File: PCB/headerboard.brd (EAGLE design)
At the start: 100 x 80 mm, 21 parts

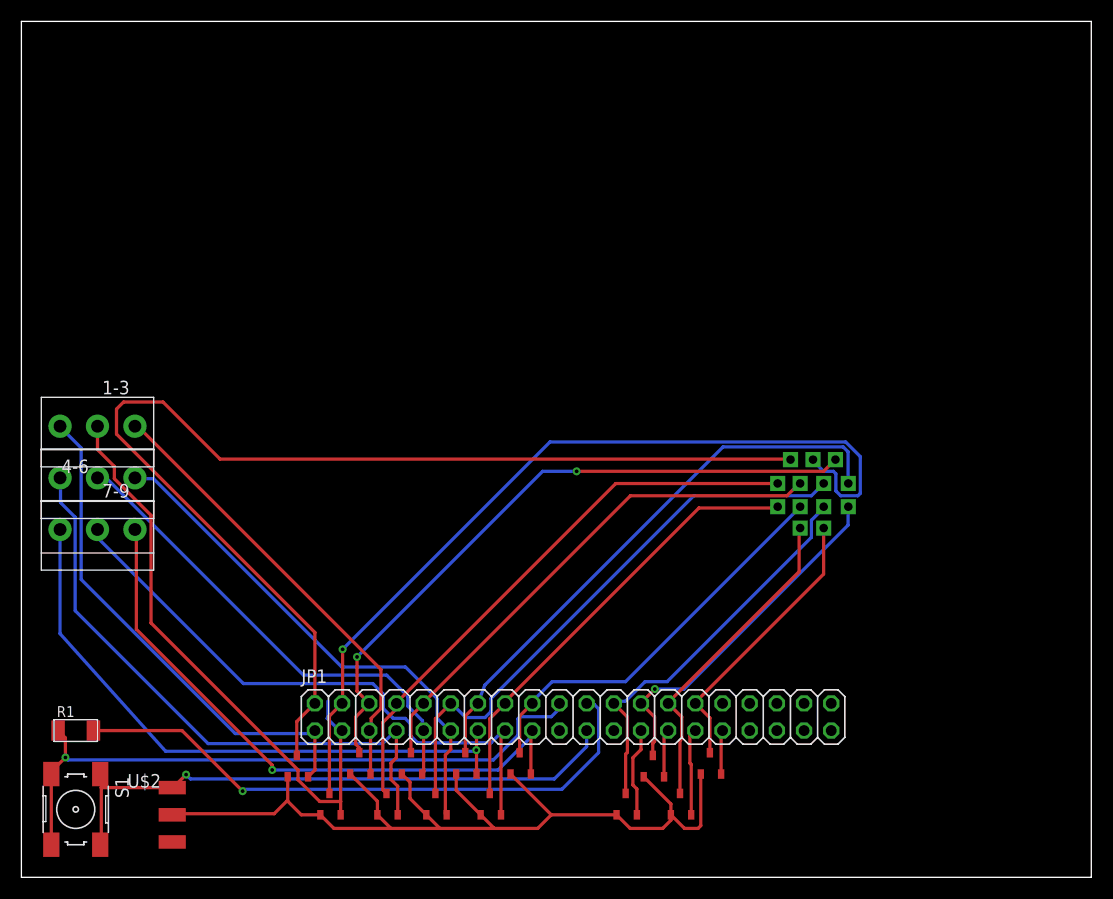
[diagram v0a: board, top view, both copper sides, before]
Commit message: Updates
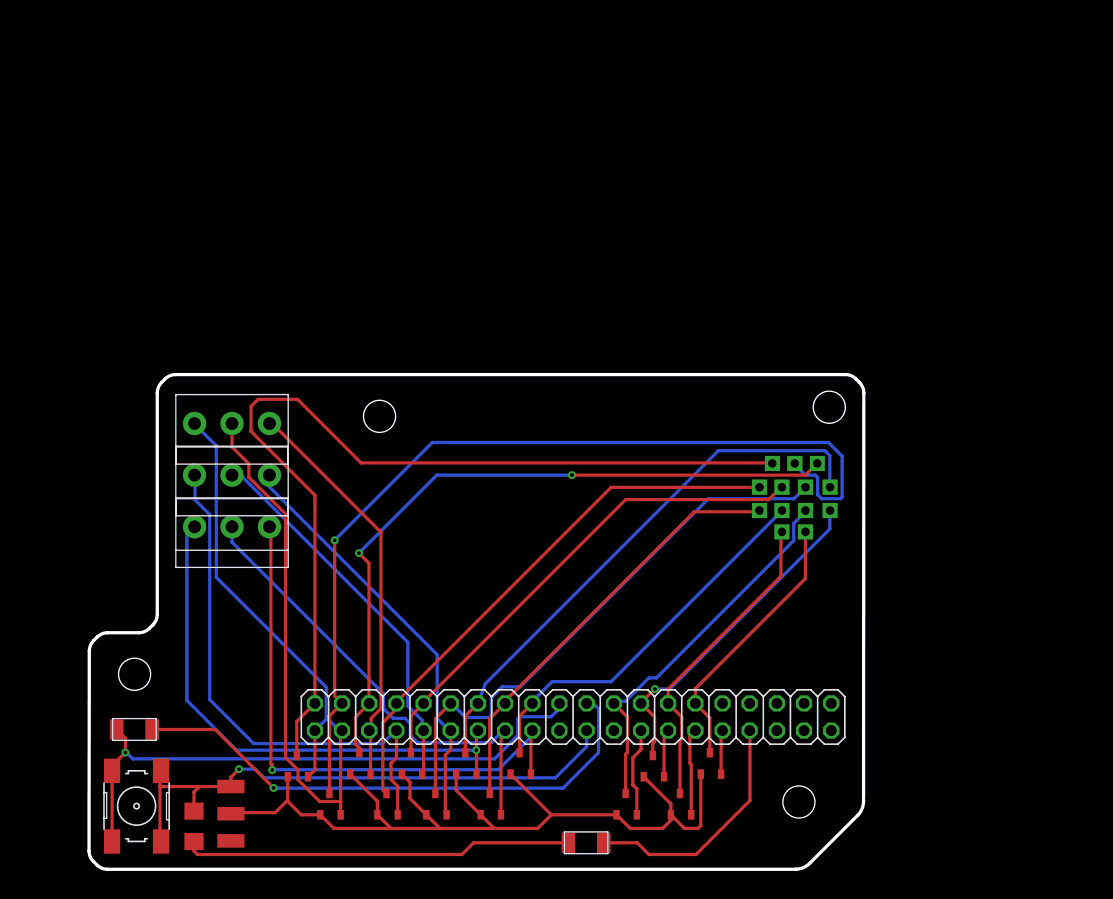
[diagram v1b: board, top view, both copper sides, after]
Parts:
- added R2: 330ohm, fab_new:R1206FAB
- added U$1: LED, eagle_fab:LED1206
- moved 1-3 12.6 mm to (19.7, 42.4)
- moved 4-6 12.6 mm to (19.7, 37.6)
- moved 7-9 12.6 mm to (19.7, 32.8)
- moved S1 5.69 mm to (10.8, 6.65)
- moved U$2 5.49 mm to (19.2, 5.94)
- moved R1 5.49 mm to (10.6, 13.8)
- moved U$19 1.74 mm to (67.4, 31.1)
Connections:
- new net N$28: JP1.33, R2.1
- new net N$29: R2.2, U$1.1
- net GND: now also U$1.2
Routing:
- net N$29: track 0.00 -> 36.5 mm
- net N$28: track 0.00 -> 22.8 mm
- net N$2: track 106.2 -> 87.3 mm
- net N$22: track 56.9 -> 44.8 mm
- net N$18: track 45.5 -> 36.0 mm
- net N$19: track 48.5 -> 39.6 mm
- net N$37: track 47.6 -> 38.8 mm
- net N$20: track 57.7 -> 49.8 mm
- net N$17: track 57.0 -> 49.6 mm
- net VCC: track 56.5 -> 50.8 mm
- net N$16: track 61.3 -> 55.6 mm
- net N$3: track 81.3 -> 86.8 mm
- net N$1: track 90.4 -> 84.9 mm
- net N$11: track 57.1 -> 52.1 mm
- net N$23: track 58.2 -> 53.2 mm
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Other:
- board size 100 x 80 mm -> 72.4 x 46.2 mm
